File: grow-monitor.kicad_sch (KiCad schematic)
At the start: 68 parts, among them J1 PH 2.0, J2 I2C1, J3 DS18B20, M1 M5StampS3, M2 AHT21B, P1 PCB_Patch, Q1 AO3401A, Q2 ALS-PT19-315C, Q3 AO3401A, Q4 2N7002, SW1 PWR2, SW2 CALIB, SW3 EN, SW4 PROG, SW5 KILL, SW6 PWR1, T1 Tooling, U1 SPX3819M5-L-3-3, U2 TPL5110, U4 DS18B20, U5 NE555P

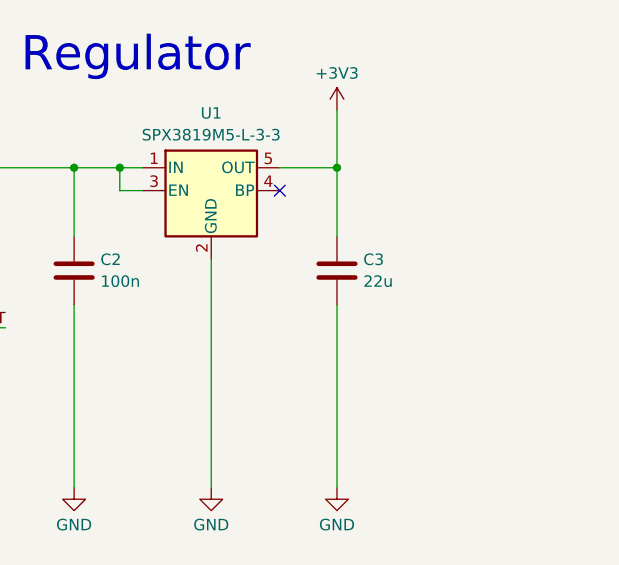
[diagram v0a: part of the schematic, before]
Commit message: Add caps
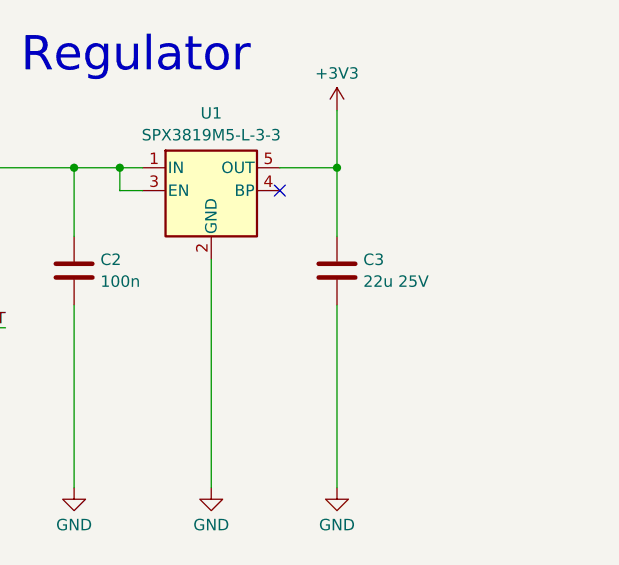
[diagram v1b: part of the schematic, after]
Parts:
- C3: value 22u -> 22u 25V; LCSC (none) -> C45783
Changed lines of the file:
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@@
 			)
 		)
-		(property "Value" "22u"
+		(property "Value" "22u 25V"
 			(at 251.841 46.9321 0)
 			(effects
@@
 			)
 		)
-		(property "LCSC" ""
+		(property "LCSC" "C45783"
 			(at 248.92 45.72 0)
 			(effects
